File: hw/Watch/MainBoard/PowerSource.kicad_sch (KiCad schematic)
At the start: 22 parts, among them J2 Conn_01x02, Q1 Q_PMOS_DGS-L, Q2 PMOS-2x_BSS84DW, Q7 PMOS-2x_BSS84DW, SW4 ON, U2 SL8261D-G3JE

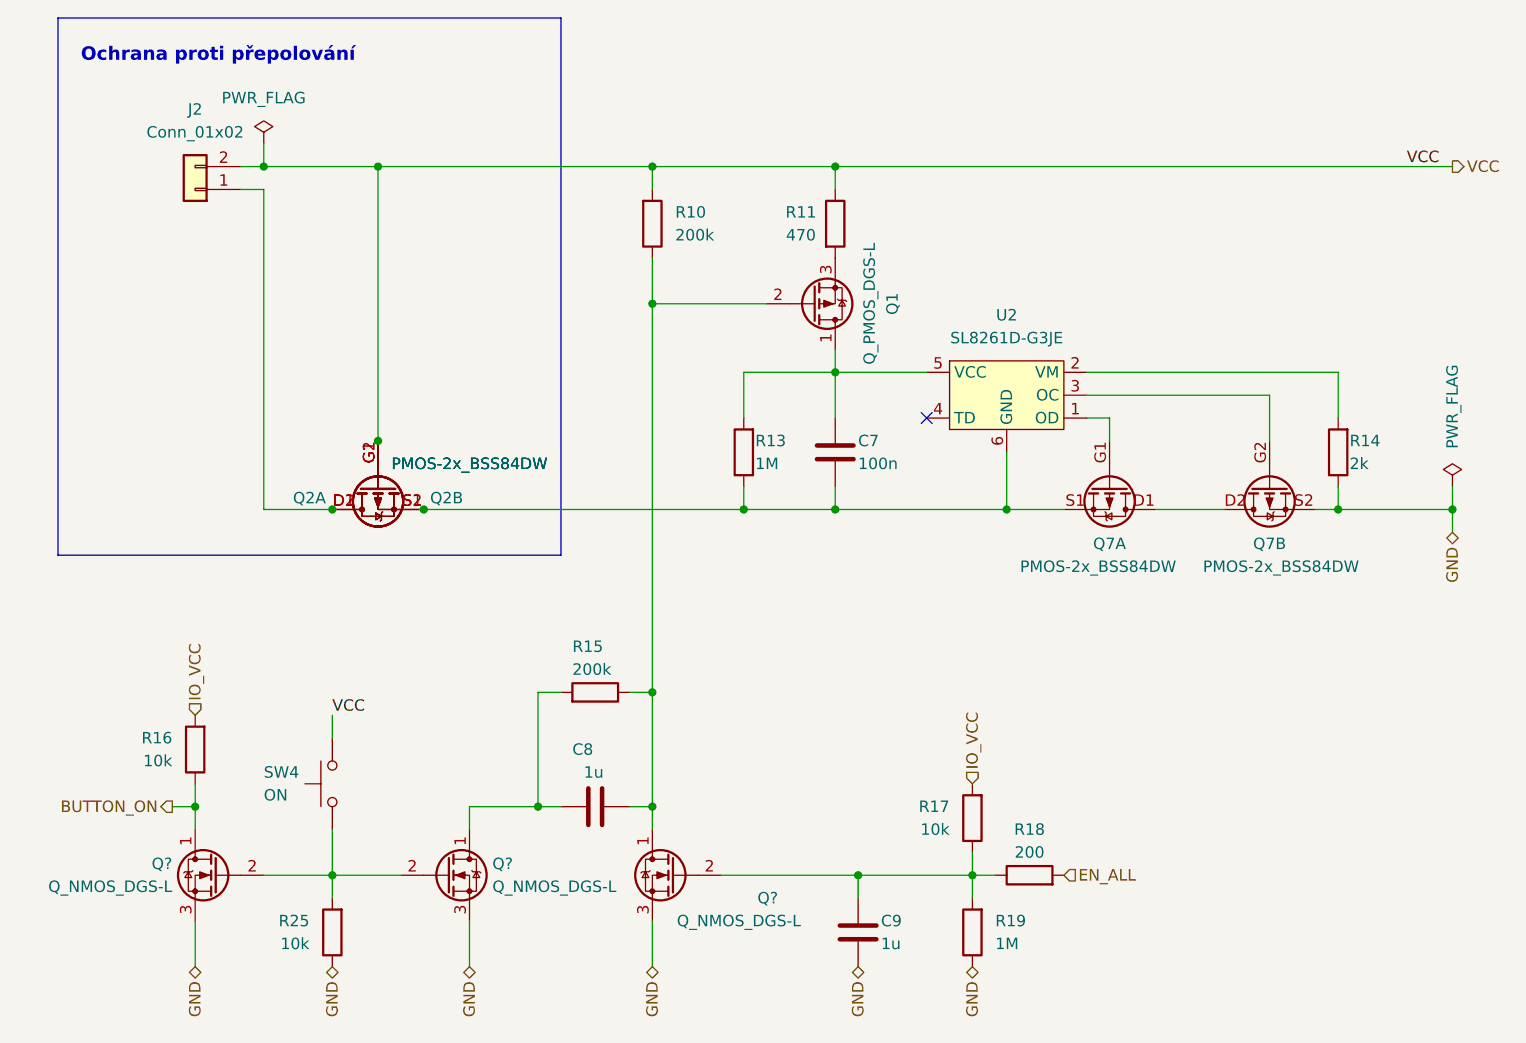
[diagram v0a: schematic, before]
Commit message: wip
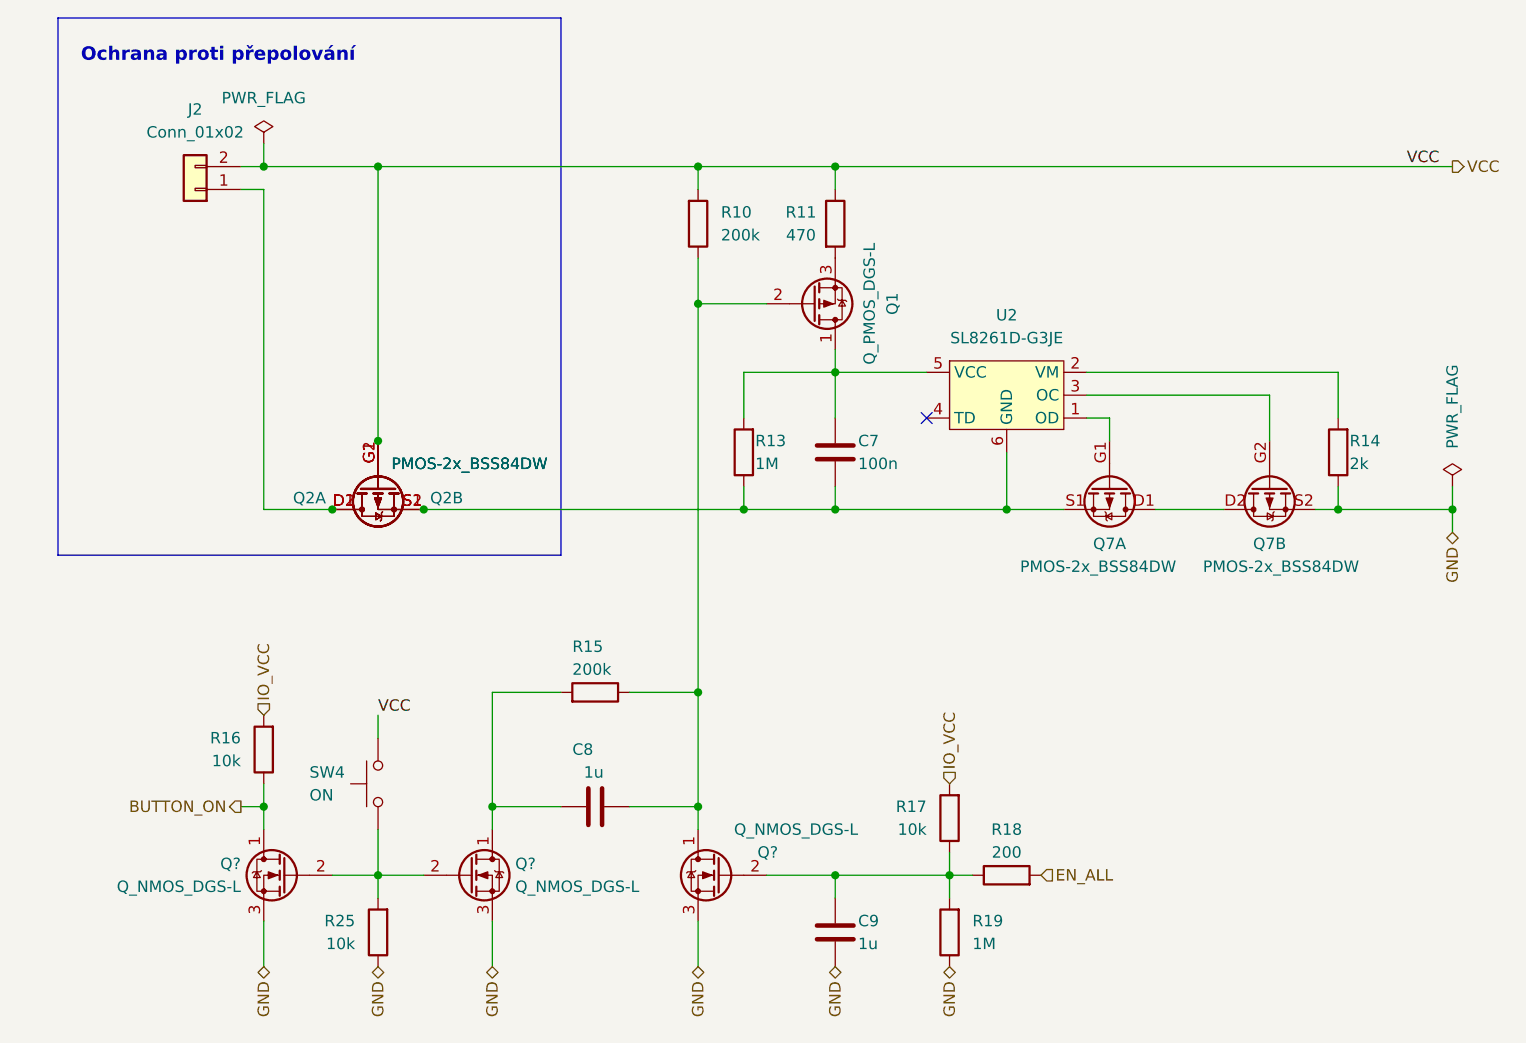
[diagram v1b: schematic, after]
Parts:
- C7: footprint Capacitor_SMD:C_0402_1005Metric -> Capacitor_SMD:C_0201_0603Metric; Basic/Extended B -> E; LCSC C307331 -> C5142565; info 50V, X7R -> 10V, X5R
- C8, C9: footprint Capacitor_SMD:C_0402_1005Metric -> Capacitor_SMD:C_0201_0603Metric; JLCPCB_CORRECTION 0;0;0 -> (none); LCSC C1518208 -> C76935; info 50V, X5R (potenciálně C52923 což je 25V, X5R ) -> 10V, X5R
- J2: footprint Connector_JST:JST_PH_S2B-PH-SM4-TB_1x02-1MP_P2.00mm_Horizontal -> Connector_PinHeader_2.00mm:PinHeader_1x02_P2.00mm_Vertical
- Q2, Q7, U2: Basic/Extended (none) -> E
- R10, R15: footprint Resistor_SMD:R_0402_1005Metric -> Resistor_SMD:R_0201_0603Metric; Basic/Extended B -> E; LCSC C25764 -> C171922
- R13, R19: footprint Resistor_SMD:R_0402_1005Metric -> Resistor_SMD:R_0201_0603Metric; Basic/Extended B -> E; LCSC C26083 -> C295786
- R16, R17, R25: footprint Resistor_SMD:R_0402_1005Metric -> Resistor_SMD:R_0201_0603Metric; Basic/Extended B -> E; JLCPCB_CORRECTION 0;0;0 -> (none); LCSC C25744 -> C106225
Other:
- moved on the sheet: C9, Q?, R10, R16, R17, R18, R19, R25, SW4
